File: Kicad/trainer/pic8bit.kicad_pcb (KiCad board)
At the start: 2 copper layers, 160 x 100 mm, 128 parts, among them K101 AC/DC 9-12V, K102 AC/DC 9-12V, K103 PE-450-4X6X-BLACK, K201 MCU 1, K202 MCU 2, K203 ICSP, K204 VIN, K205 VIN, K206 VDD, K207 GND, K208 VDD, K209 GND, K210 SYMBOL-HEADER-F-1X10, K301 I2C/GPIO, K302 I2C/SPI, K303 SPI/GPIO, K304 EUSART/TTL, K402 SYMBOL-HEADER-F-1X10, K409 HARWIN-254-F-1X16-VERTICAL, K410 LED, P401 AN1, P402 AN2, U101 KEYSTONE-24283, U102 KEYSTONE-24283, U103 KEYSTONE-24283, U104 KEYSTONE-24283, U105 NCP5662-ADJ-TO263, U201 MICROCHIP-PIC16F1778-ISP, X1 XTAL-DIL08, X101 3M-SJ5376, X102 3M-SJ5376, X103 3M-SJ5376, X104 3M-SJ5376, X105 3M-SJ5376

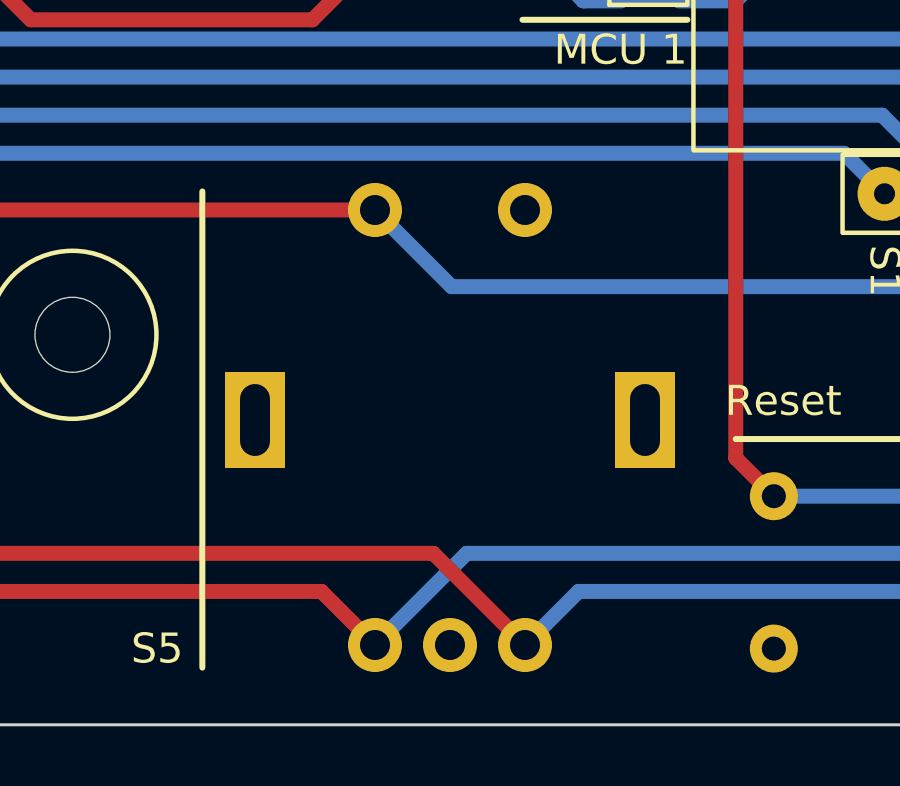
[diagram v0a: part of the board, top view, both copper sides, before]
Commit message: Update
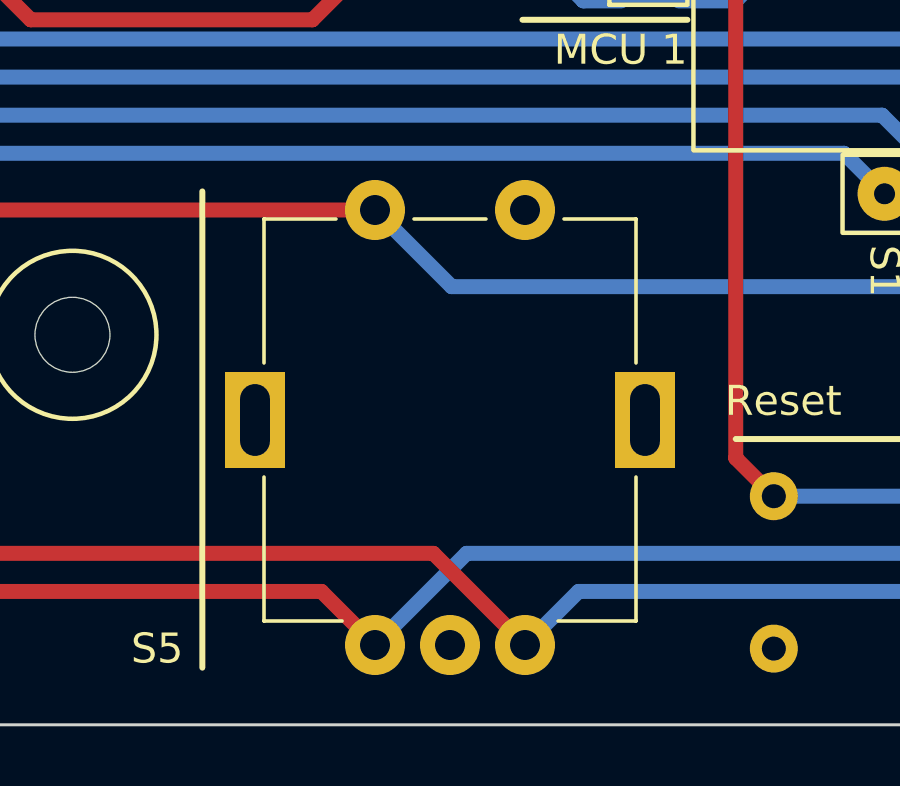
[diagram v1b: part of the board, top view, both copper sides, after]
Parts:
- S403: footprint tronixio:BOURNS-PEC12R -> tronixio:BOURNS-PEC12R-SWITCH
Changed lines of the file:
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@@
     )
   )
-  (footprint "tronixio:BOURNS-PEC12R" (layer "F.Cu")
+  (footprint "tronixio:BOURNS-PEC12R-SWITCH" (layer "F.Cu")
     (at 175.585 136.84)
+    (descr "https://www.bourns.com/resources/design-tools/engineering-files-list?Folder=PEC12R")
     (property "Mouser" "652-PEC12R-4215F-S24")
     (property "Sheetfile" "pic8bit-hid.kicad_sch")
     (property "Sheetname" "HID")
     (attr through_hole)
-    (fp_text reference "S403" (at 0 -5) (layer "F.Fab")
+    (fp_text reference "S403" (at 0 -10.16) (layer "F.Fab")
       (effects (font (size 1 1) (thickness 0.15)))
     )
-    (fp_text value "BOURNS-PEC12R-24DENTS" (at 0 -9) (layer "F.Fab")
+    (fp_text value "BOURNS-PEC12R-24DENTS" (at 0 10.16) (layer "F.Fab")
       (effects (font (size 1 1) (thickness 0.15)))
     )
+    (fp_line (start -6.2 6.7) (end -3.6 6.7) (layer "F.SilkS") (width 0.12))
+    (fp_line (start 3.8 -6.7) (end 6.2 -6.7) (layer "F.SilkS") (width 0.12))
+    (fp_line (start 6.2 -6.7) (end 6.2 -1.9) (layer "F.SilkS") (width 0.12))
+    (fp_line (start -6.2 -6.7) (end -3.8 -6.7) (layer "F.SilkS") (width 0.12))
+    (fp_line (start -6.2 1.9) (end -6.2 6.7) (layer "F.SilkS") (width 0.12))
+    (fp_line (start -6.2 -6.7) (end -6.2 -1.9) (layer "F.SilkS") (width 0.12))
+    (fp_line (start 3.6 6.7) (end 6.2 6.7) (layer "F.SilkS") (width 0.12))
+    (fp_line (start 6.2 1.9) (end 6.2 6.7) (layer "F.SilkS") (width 0.12))
+    (fp_line (start -1.2 -6.7) (end 1.2 -6.7) (layer "F.SilkS") (width 0.12))
     (fp_rect (start -7.7 8.6) (end 7.7 -8.1) (layer "F.CrtYd") (width 0.05) (fill none))
     (fp_line (start -2 1.5) (end -1.8 1) (layer "F.Fab") (width 0.1))
+    (fp_line (start -1.8 1) (end 1.8 1) (layer "F.Fab") (width 0.1))
     (fp_line (start 2 1.5) (end 1.8 1) (layer "F.Fab") (width 0.1))
     (fp_line (start -2 1.5) (end 2 1.5) (layer "F.Fab") (width 0.1))
-    (fp_line (start -1.8 1) (end 1.8 1) (layer "F.Fab") (width 0.1))
+    (fp_rect (start -3 7.1) (end -2 6.7) (layer "F.Fab") (width 0.1) (fill solid))
+    (fp_rect (start 6.2 1.25) (end 7 -1.25) (layer "F.Fab") (width 0.1) (fill solid))
+    (fp_rect (start -6.2 6.7) (end 6.2 -6.7) (layer "F.Fab") (width 0.1) (fill none))
+    (fp_rect (start -3 -6.7) (end -2 -7.1) (layer "F.Fab") (width 0.1) (fill solid))
+    (fp_rect (start 2 7.1) (end 3 6.7) (layer "F.Fab") (width 0.1) (fill solid))
     (fp_rect (start -0.5 7.1) (end 0.5 6.7) (layer "F.Fab") (width 0.1) (fill solid))
-    (fp_rect (start -3 7.1) (end -2 6.7) (layer "F.Fab") (width 0.1) (fill solid))
-    (fp_rect (start -6.2 6.7) (end 6.2 -6.7) (layer "F.Fab") (width 0.1) (fill none))
     (fp_rect (start -7 1.25) (end -6.2 -1.25) (layer "F.Fab") (width 0.1) (fill solid))
-    (fp_rect (start 6.2 1.25) (end 7 -1.25) (layer "F.Fab") (width 0.1) (fill solid))
-    (fp_rect (start 2 7.1) (end 3 6.7) (layer "F.Fab") (width 0.1) (fill solid))
     (fp_rect (start 2 -6.7) (end 3 -7.1) (layer "F.Fab") (width 0.1) (fill solid))
-    (fp_rect (start -3 -6.7) (end -2 -7.1) (layer "F.Fab") (width 0.1) (fill solid))
     (fp_arc (start -1.8 1) (mid 0 -2.046667) (end 1.8 1) (layer "F.Fab") (width 0.1))
     (fp_circle (center 5.3 6) (end 5.6 6) (layer "F.Fab") (width 0.1) (fill none))
     (fp_circle (center 5.3 -5.5) (end 5.6 -5.5) (layer "F.Fab") (width 0.1) (fill none))
+    (fp_circle (center -5.3 -5.5) (end -5 -5.5) (layer "F.Fab") (width 0.1) (fill none))
+    (fp_circle (center -5.3 6) (end -5 6) (layer "F.Fab") (width 0.1) (fill none))
+    (fp_circle (center 0 0) (end 2.5 0) (layer "F.Fab") (width 0.1) (fill none))
     (fp_circle (center 0 0) (end 3.5 0) (layer "F.Fab") (width 0.1) (fill none))
-    (fp_circle (center 0 0) (end 2.5 0) (layer "F.Fab") (width 0.1) (fill none))
-    (fp_circle (center -5.3 6) (end -5 6) (layer "F.Fab") (width 0.1) (fill none))
-    (fp_circle (center -5.3 -5.5) (end -5 -5.5) (layer "F.Fab") (width 0.1) (fill none))
-    (pad "1" thru_hole circle locked (at -2.5 7.5) (size 1.8 1.8) (drill 1) (layers *.Cu *.Mask)
+    (pad "1" thru_hole circle (at -2.5 7.5) (size 2 2) (drill 1) (layers *.Cu *.Mask)
       (net 105 "/HID/A") (pinfunction "A") (pintype "passive"))
-    (pad "2" thru_hole rect locked (at -6.5 0) (size 2 3.2) (drill oval 1 2.4) (layers *.Cu *.Mask)
-      (net 1 "GND") (pinfunction "C") (pintype "passive"))
-    (pad "2" thru_hole circle locked (at 0 7.5) (size 1.8 1.8) (drill 1) (layers *.Cu *.Mask)
-      (net 1 "GND") (pinfunction "C") (pintype "passive"))
-    (pad "2" thru_hole rect locked (at 6.5 0) (size 2 3.2) (drill oval 1 2.4) (layers *.Cu *.Mask)
-      (net 1 "GND") (pinfunction "C") (pintype "passive"))
-    (pad "3" thru_hole circle locked (at 2.5 7.5) (size 1.8 1.8) (drill 1) (layers *.Cu *.Mask)
+    (pad "2" thru_hole circle (at 0 7.5) (size 2 2) (drill 1) (layers *.Cu *.Mask)
+      (net 1 "GND") (pintype "passive"))
+    (pad "2" thru_hole rect (at 6.5 0) (size 2 3.2) (drill oval 1 2.4) (layers *.Cu *.Mask)
+      (net 1 "GND") (pintype "passive"))
+    (pad "2" thru_hole rect (at -6.5 0) (size 2 3.2) (drill oval 1 2.4) (layers *.Cu *.Mask)
+      (net 1 "GND") (pintype "passive"))
+    (pad "3" thru_hole circle (at 2.5 7.5) (size 2 2) (drill 1) (layers *.Cu *.Mask)
       (net 106 "/HID/B") (pinfunction "B") (pintype "passive"))
-    (pad "4" thru_hole circle locked (at 2.5 -7) (size 1.8 1.8) (drill 1) (layers *.Cu *.Mask)
-      (net 1 "GND") (pinfunction "2") (pintype "passive"))
-    (pad "5" thru_hole circle locked (at -2.5 -7) (size 1.8 1.8) (drill 1) (layers *.Cu *.Mask)
-      (net 99 "/HID/S5") (pinfunction "1") (pintype "passive"))
-    (model "${KICAD6_USER_3DMODEL_DIR}/Discret/BOURNS-PEC12R.step"
+    (pad "4" thru_hole circle (at 2.5 -7) (size 2 2) (drill 1) (layers *.Cu *.Mask)
+      (net 1 "GND") (pintype "passive"))
+    (pad "5" thru_hole circle (at -2.5 -7) (size 2 2) (drill 1) (layers *.Cu *.Mask)
+      (net 99 "/HID/S5") (pintype "passive"))
+    (model "${KICAD6_USER_3DMODEL_DIR}/Switch/BOURNS-PEC12R-SWITCH.step"
       (offset (xyz 0 0 0))
       (scale (xyz 1 1 1))
